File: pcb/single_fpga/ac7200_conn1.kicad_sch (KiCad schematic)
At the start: 1 part, among them U97 ALINX AC7200 (XC7A200T-2FBG48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

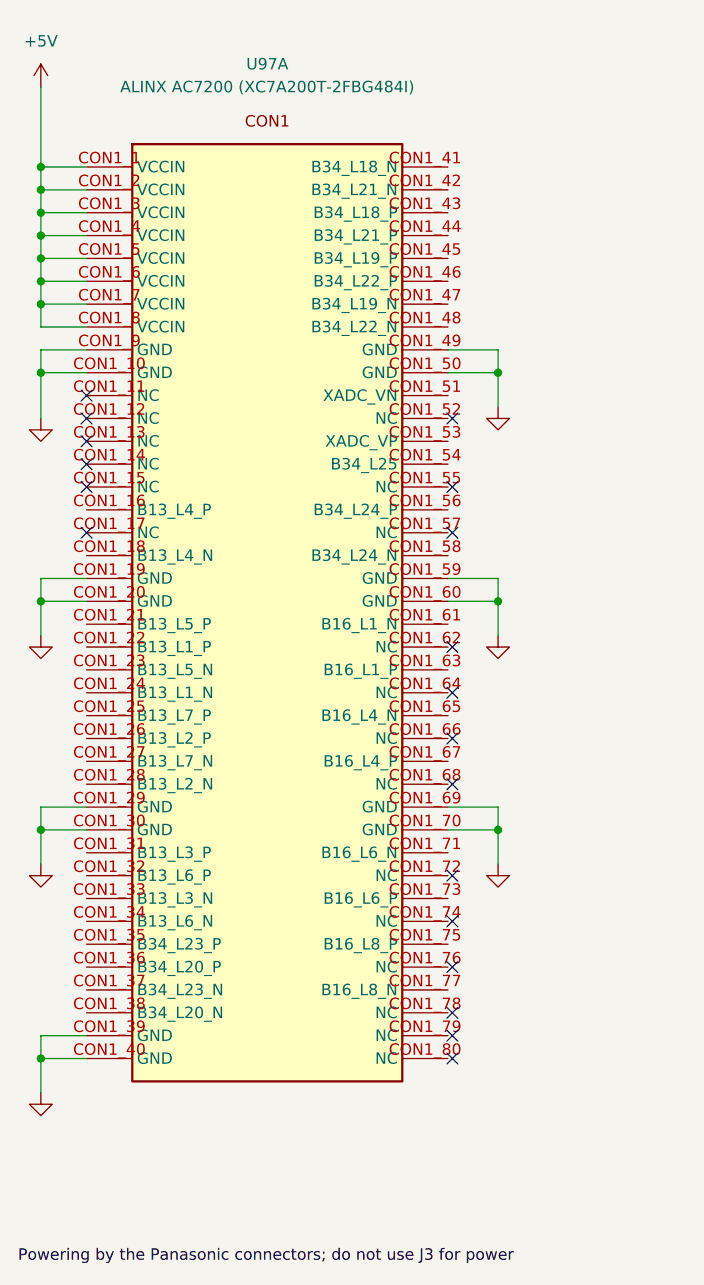
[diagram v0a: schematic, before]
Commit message: Fixed.
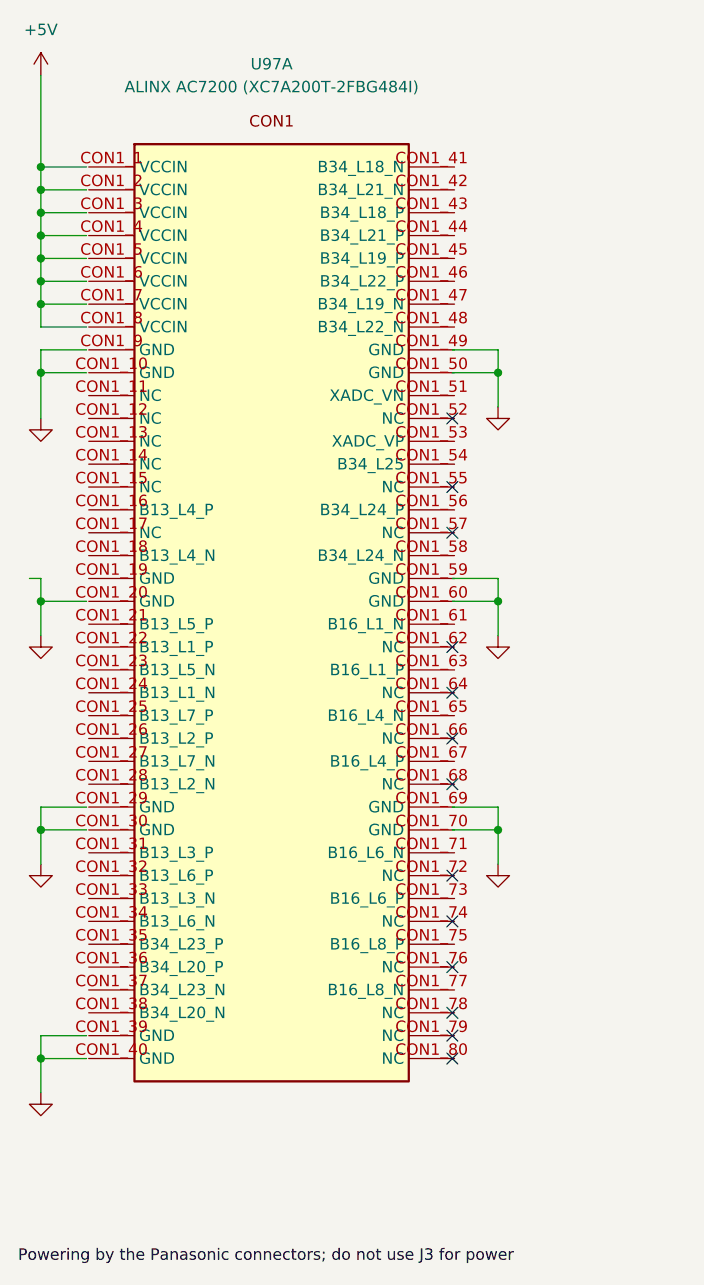
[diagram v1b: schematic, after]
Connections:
- net +5V: no longer U97.CON1_1 (VCCIN), U97.CON1_2 (VCCIN), U97.CON1_3 (VCCIN), U97.CON1_4 (VCCIN), U97.CON1_5 (VCCIN), U97.CON1_6 (VCCIN), U97.CON1_7 (VCCIN), U97.CON1_8 (VCCIN)
- net GND: no longer U97.CON1_10 (GND), U97.CON1_19 (GND), U97.CON1_20 (GND), U97.CON1_29 (GND), U97.CON1_30 (GND), U97.CON1_39 (GND), U97.CON1_40 (GND), U97.CON1_49 (GND), U97.CON1_50 (GND), U97.CON1_59 (GND), U97.CON1_60 (GND), U97.CON1_69 (GND), U97.CON1_70 (GND), U97.CON1_9 (GND)
- no-connect marks 19 -> 13
